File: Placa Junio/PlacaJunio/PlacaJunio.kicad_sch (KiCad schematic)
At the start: 13 parts, among them IC1 LC86LICMD, J1 Bateria, Q4 IRLML0030, U4 MODULO MICRO SD, U5 TSR2-2433N

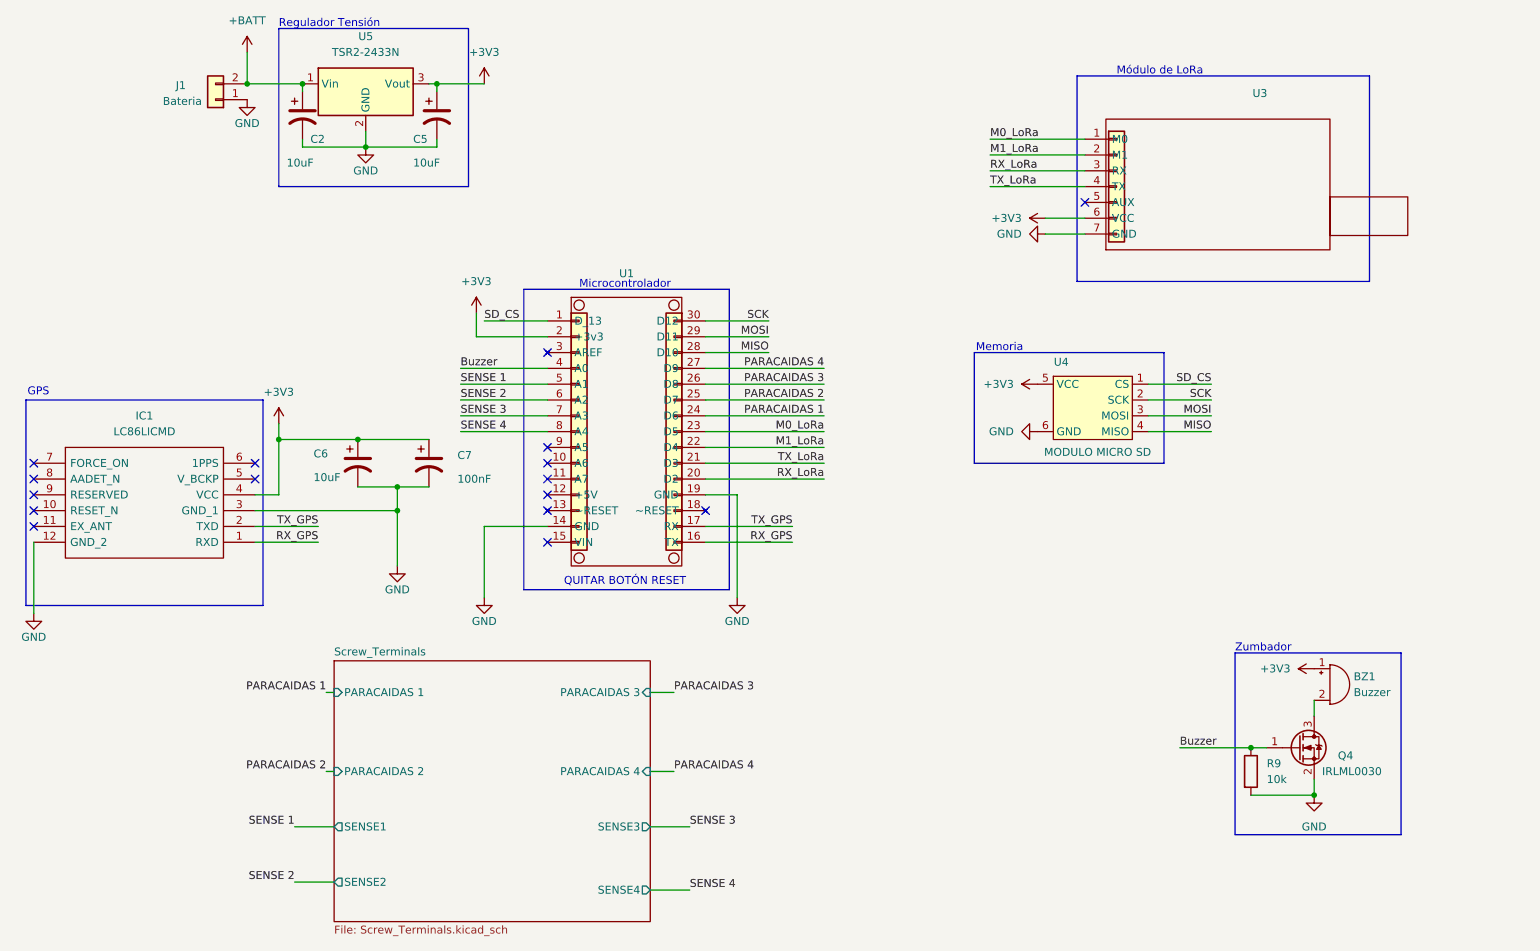
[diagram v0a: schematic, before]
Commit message: cj
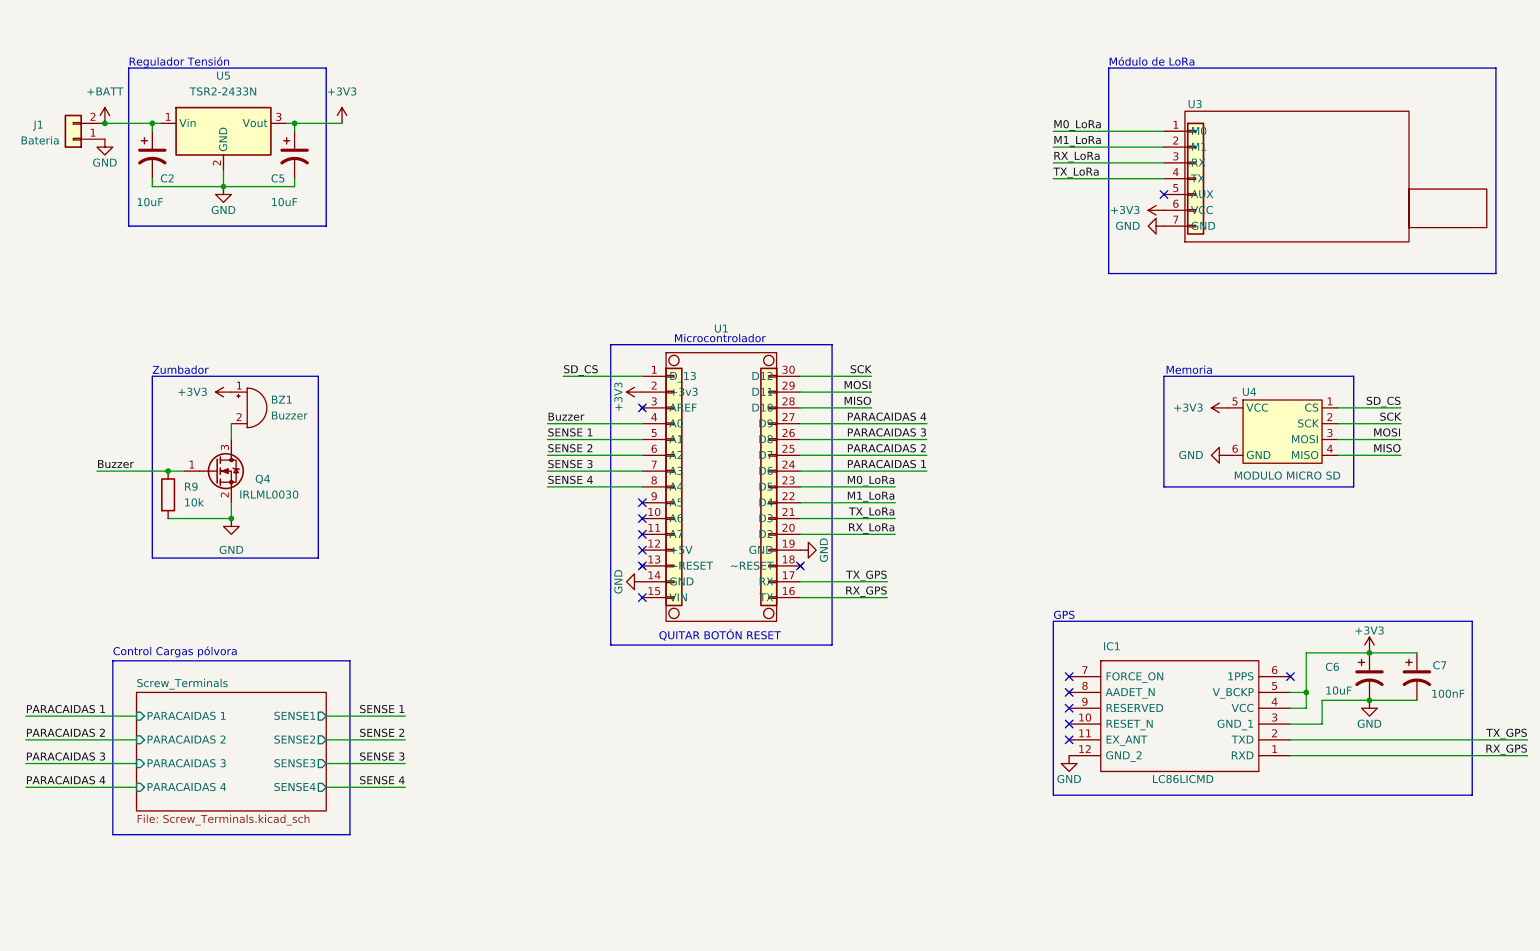
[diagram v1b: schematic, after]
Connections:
- net +3V3: now also IC1.5 (V_BCKP)
- no-connect marks 16 -> 15
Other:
- note added: "Control Cargas pólvora"
- moved on the sheet: BZ1, C2, C5, C6, C7, IC1, J1, Q4, R9, U1, U3, U4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
